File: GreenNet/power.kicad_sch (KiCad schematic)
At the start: 1 part, among them U5 MC33063AD

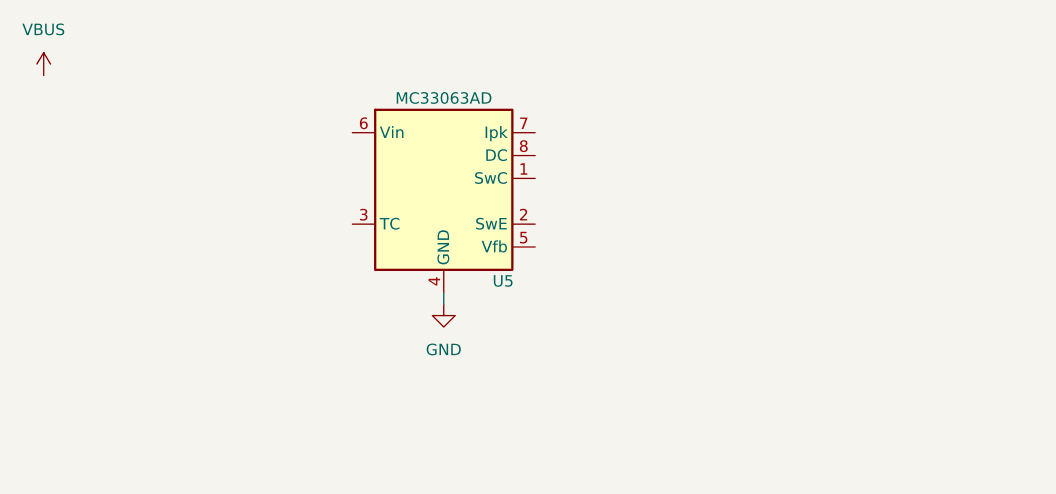
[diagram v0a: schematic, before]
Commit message: USB-PC PD progress
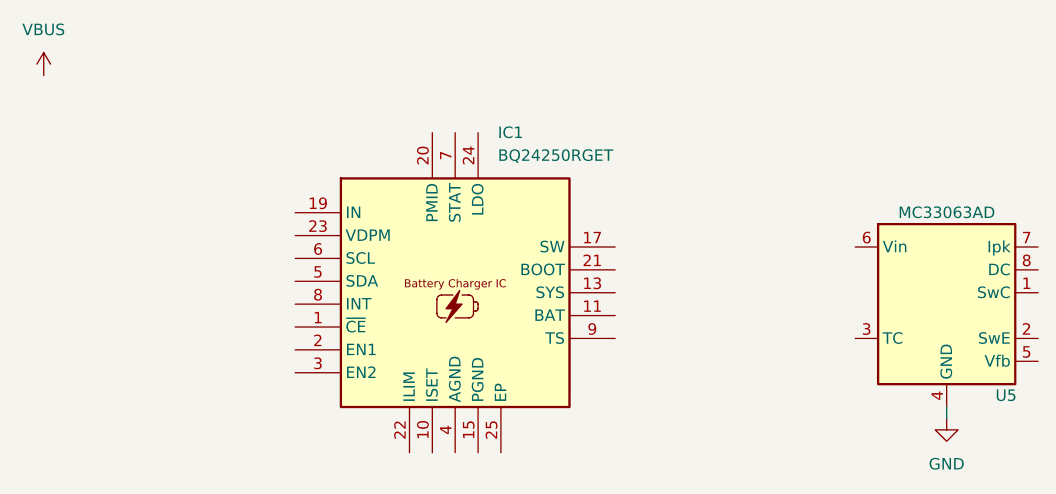
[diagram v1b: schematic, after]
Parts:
- added IC1: BQ24250RGET, QFN50P400X400X100-25N-D, symbol AA_Power_ICs:BQ24250RGET
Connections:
- new net: IC1.11 (BAT), IC1.12 (BAT)
- new net: IC1.13 (SYS), IC1.14 (SYS)
- new net: IC1.15 (PGND), IC1.16 (PGND)
- new net: IC1.17 (SW), IC1.18 (SW)
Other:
- moved on the sheet: U5
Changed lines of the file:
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@@
 	(wire
 		(pts
-			(xy 107.95 86.36) (xy 107.95 87.63)
+			(xy 163.83 99.06) (xy 163.83 100.33)
 		)
 		(stroke
@@
 	(symbol
 		(lib_id "power:GND")
-		(at 107.95 87.63 0)
+		(at 163.83 100.33 0)
 		(unit 1)
 		(exclude_from_sim no)
@@
 		(fields_autoplaced yes)
 		(property "Reference" "#PWR036"
-			(at 107.95 93.98 0)
+			(at 163.83 106.68 0)
 			(effects
 				(font
@@
 		)
 		(property "Value" "GND"
-			(at 107.95 92.71 0)
+			(at 163.83 105.41 0)
 			(effects
 				(font
@@
 		)
 		(property "Footprint" ""
-			(at 107.95 87.63 0)
+			(at 163.83 100.33 0)
 			(effects
 				(font
@@
 		)
 		(property "Datasheet" ""
-			(at 107.95 87.63 0)
+			(at 163.83 100.33 0)
 			(effects
 				(font
@@
 		)
 		(property "Description" "Power symbol creates a global label with name \"GND\" , ground"
-			(at 107.95 87.63 0)
+			(at 163.83 100.33 0)
 			(effects
 				(font
@@
 	)
 	(symbol
+		(lib_id "AA_Power_ICs:BQ24250RGET")
+		(at 109.22 86.36 0)
+		(unit 1)
+		(exclude_from_sim no)
+		(in_bom yes)
+		(on_board yes)
+		(dnp no)
+		(fields_autoplaced yes)
+		(property "Reference" "IC1"
+			(at 113.9541 68.58 0)
+			(effects
+				(font
+					(size 1.27 1.27)
+				)
+				(justify left)
+			)
+		)
+		(property "Value" "BQ24250RGET"
+			(at 113.9541 71.12 0)
+			(effects
+				(font
+					(size 1.27 1.27)
+				)
+				(justify left)
+			)
+		)
+		(property "Footprint" "QFN50P400X400X100-25N-D"
+			(at 156.464 73.406 0)
+			(effects
+				(font
+					(size 1.27 1.27)
+				)
+				(justify left top)
+				(hide yes)
+			)
+		)
+		(property "Datasheet" "https://www.ti.com/lit/ds/symlink/bq24250.pdf"
+			(at 156.464 77.724 0)
+			(effects
+				(font
+					(size 1.27 1.27)
+				)
+				(justify left top)
+				(hide yes)
+			)
+		)
+		(property "Description" "2A Single Input I2C/Standalone Switch-Mode Li-Ion Battery Charger"
+			(at 190.246 76.2 0)
+			(effects
+				(font
+					(size 1.27 1.27)
+				)
+				(hide yes)
+			)
+		)
+		(property "Height" "1"
+			(at 135.89 473.66 0)
+			(effects
+				(font
+					(size 1.27 1.27)
+				)
+				(justify left top)
+				(hide yes)
+			)
+		)
+		(property "Manufacturer_Name" "Texas Instruments"
+			(at 156.464 71.12 0)
+			(effects
+				(font
+					(size 1.27 1.27)
+				)
+				(justify left top)
+				(hide yes)
+			)
+		)
+		(pin "16"
+		)
+		(pin "12"
+		)
+		(pin "8"
+		)
+		(pin "21"
+		)
+		(pin "5"
+		)
+		(pin "10"
+		)
+		(pin "14"
+		)
+		(pin "18"
+		)
+		(pin "7"
+		)
+		(pin "2"
+		)
+		(pin "19"
+		)
+		(pin "15"
+		)
+		(pin "20"
+		)
+		(pin "13"
+		)
+		(pin "3"
+		)
+		(pin "6"
+		)
+		(pin "4"
+		)
+		(pin "1"
+		)
+		(pin "22"
+		)
+		(pin "9"
+		)
+		(pin "25"
+		)
+		(pin "11"
+		)
+		(pin "23"
+		)
+		(pin "17"
+		)
+		(pin "24"
+		)
+		(instances
+			(project ""
+				(path "/189669a5-f2fc-4cde-9413-8df80c557655/25a95746-0a87-4e99-99e5-3474e5066d9d"
+					(reference "IC1")
+					(unit 1)
+				)
+			)
+		)
+	)
+	(symbol
 		(lib_id "Regulator_Switching:MC33063AD")
-		(at 107.95 73.66 0)
+		(at 163.83 86.36 0)
 		(unit 1)
 		(exclude_from_sim no)
@@
 		(dnp no)
 		(property "Reference" "U5"
-			(at 114.554 85.09 0)
+			(at 170.434 97.79 0)
 			(effects
 				(font
@@
 		)
 		(property "Value" "MC33063AD"
-			(at 107.95 64.77 0)
+			(at 163.83 77.47 0)
 			(effects
 				(font
@@
 		)
 		(property "Footprint" "Package_SO:SOIC-8_3.9x4.9mm_P1.27mm"
-			(at 109.22 85.09 0)
+			(at 165.1 97.79 0)
 			(effects
 				(font
@@
 		)
 		(property "Datasheet" "http://www.onsemi.com/pub_link/Collateral/MC34063A-D.PDF"
-			(at 120.65 76.2 0)
+			(at 176.53 88.9 0)
 			(effects
 				(font
@@
 		)
 		(property "Description" "1.5A, step-up/down/inverting switching regulator, 3-40V Vin, 100kHz, SO-8"
-			(at 107.95 73.66 0)
-			(effects
-				(font
+			(at 163.83 86.36 0)
+			(effects
+				(font

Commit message: started layout
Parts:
- IC1: footprint QFN50P400X400X100-25N-D -> QFN:QFN50P400X400X100-25N-D
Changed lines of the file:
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@@
 			)
 		)
-		(property "Footprint" "QFN50P400X400X100-25N-D"
+		(property "Footprint" "QFN:QFN50P400X400X100-25N-D"
 			(at 156.464 73.406 0)
 			(effects
